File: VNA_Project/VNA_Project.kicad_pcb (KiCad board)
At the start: 6 copper layers, 200 x 200 mm, 231 parts, among them J201 USB_C_Receptacle_USB2.0_16P, J202 Jack-DC, J203 Screw_Terminal_01x01, J301 2x5 1.27mm, J302 Screw_Terminal_01x02, J401 Conn_Coaxial, J402 Conn_Coaxial, J403 Conn_Coaxial, J501 RJ45_Amphenol_RJMG1BD3B8K1ANR, SW201 SW_SPDT, SW202 SW_SPDT, SW301 SW_SPDT, SW401 SW_SPDT, SW402 SW_SPDT, SW403 SW_SPDT, U201 AP63205WU, U202 AP63203WU, U203 USBLC6-2SC6, U204 HT7533-1, U205 MIC5501-3.0YM5, U206 TPS54620RGYR, U207 MCP1804x-A002xOT, U301 TMP75AID, U302 TMP75AID, U303 STM32H730VBTx, U304 TMP75AID, U305 TL972IPWR, U401 LT1813CS8-TRPBF, U402 LT1813CS8-TRPBF, U403 AD9238BSTZ-20, U404 AD8138ARZ, U405 AD8138ARZ, U501 LAN8742A, U502 USBLC6-4SC6, Y301 STDCZS1-25M, Y501 STDCZS1-25M

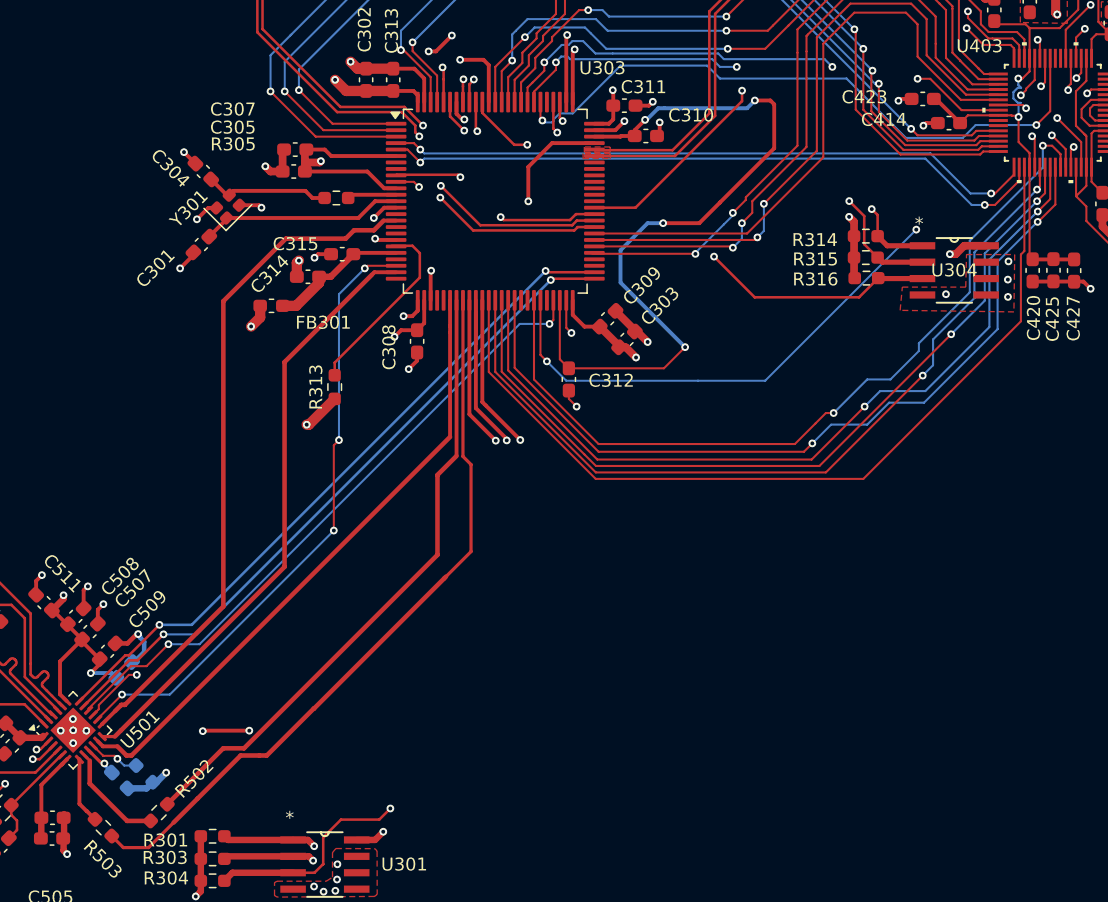
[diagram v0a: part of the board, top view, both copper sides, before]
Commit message: clearance changed
clearance changed
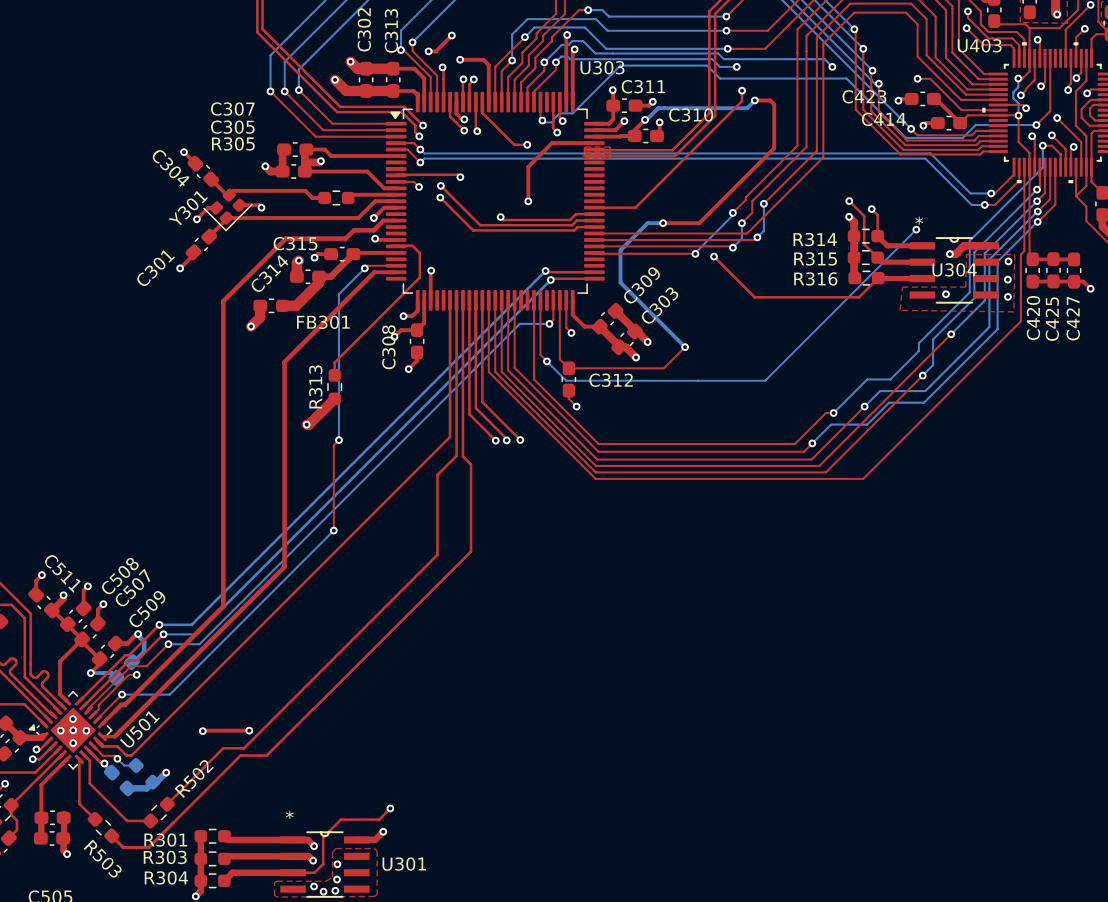
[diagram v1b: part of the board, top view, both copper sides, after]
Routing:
- net Net-(C414-Pad1): track 39.8 -> 39.1 mm
